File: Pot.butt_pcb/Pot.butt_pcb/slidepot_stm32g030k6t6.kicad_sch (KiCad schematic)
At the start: 11 parts, among them J3 Conn_01x05_Male, SW10 SW_Push, U2 STM32G030K6T6

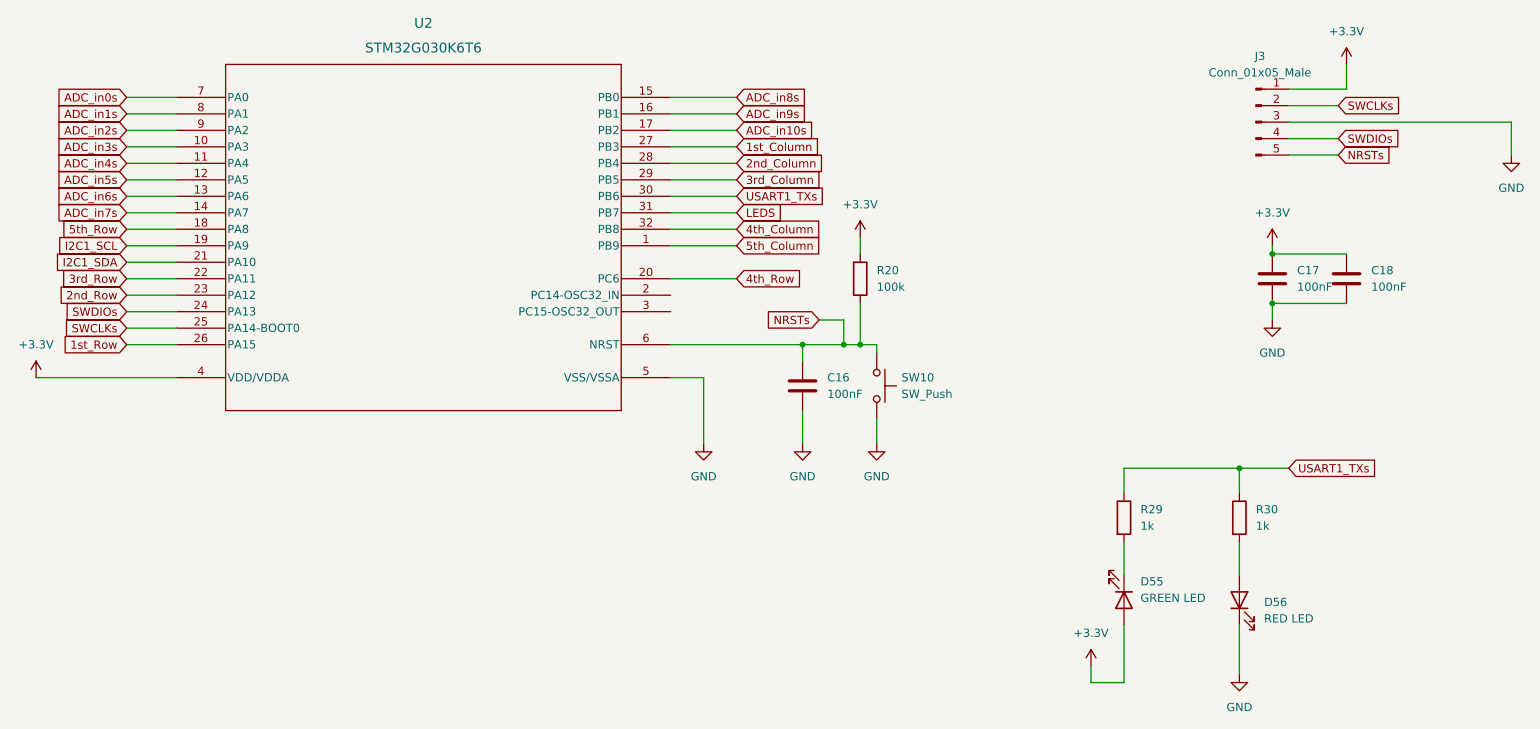
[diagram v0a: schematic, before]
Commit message: pcb design fixing
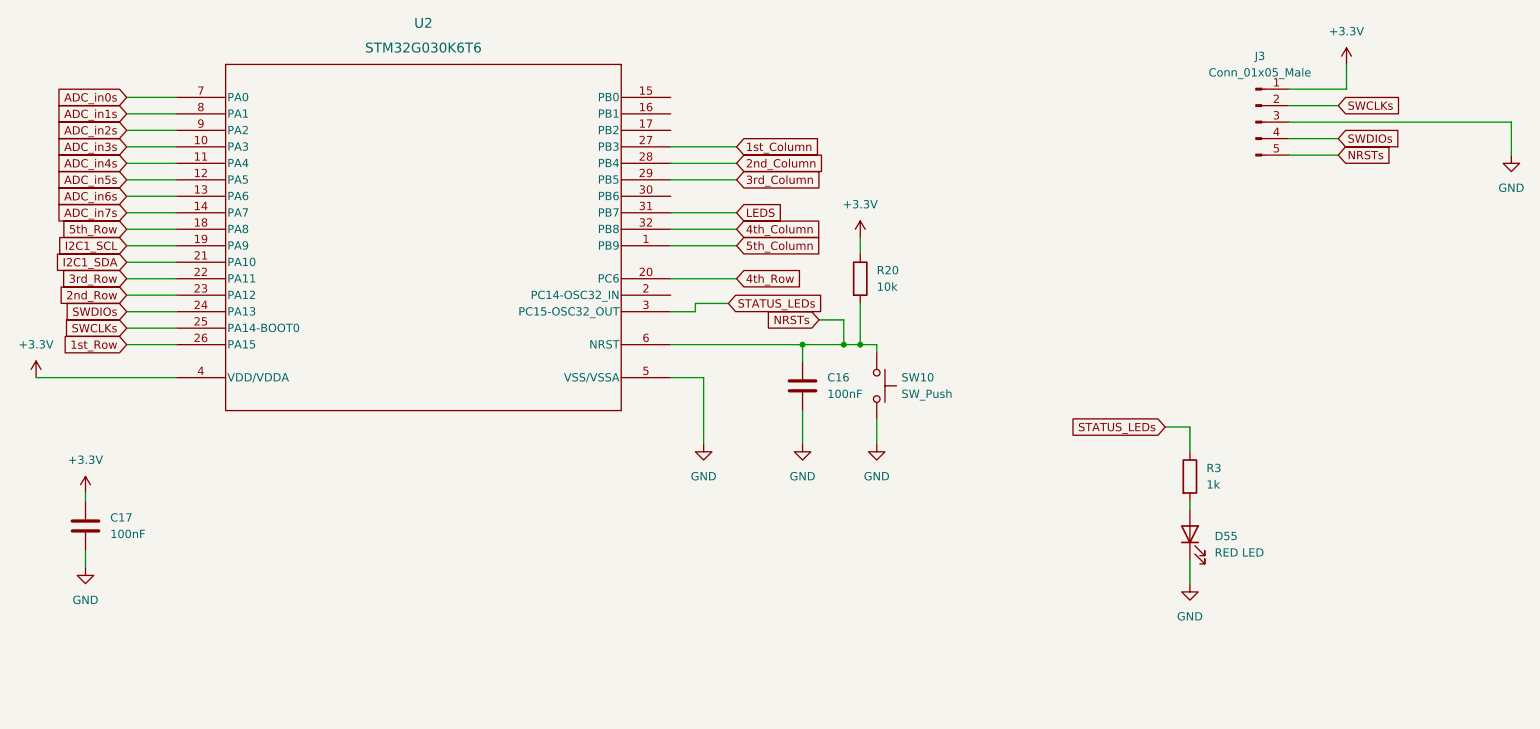
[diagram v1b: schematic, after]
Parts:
- removed C18: 100nF, Capacitor_SMD:C_0805_2012Metric_Pad1.18x1.45mm_HandSolder, symbol Device:C
- removed D56: RED LED, LED_SMD:LED_0805_2012Metric_Pad1.15x1.40mm_HandSolder, symbol Device:LED
- removed R29, R30: 1k, Resistor_SMD:R_0805_2012Metric_Pad1.20x1.40mm_HandSolder, symbol Device:R
- added R3: 1k, Resistor_SMD:R_0805_2012Metric_Pad1.20x1.40mm_HandSolder, symbol Device:R
- D55: value GREEN LED -> RED LED
- R20: value 100k -> 10k
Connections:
- net +3V3: no longer D55.2 (A)
- net GND: now also D55.1 (K)
- net STATUS_LEDs: now reaches U2.3 (PC15-OSC32_OUT)
- net STATUS_LEDs: now also R3.1
- net ADC_in10s: no longer names the net of U2.17 (PB2)
- net ADC_in8s: no longer names the net of U2.15 (PB0)
- net ADC_in9s: no longer names the net of U2.16 (PB1)
- net USART1_TXs: no longer names the net of U2.30 (PB6)
- new net: D55.2 (A), R3.2
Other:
- moved on the sheet: C17
